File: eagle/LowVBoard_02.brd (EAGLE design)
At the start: 113 x 52.1 mm, 29 parts, among them IC1 ATMEGA328P-PU, IC2 MCP7940M, IC3 SN74HC595, IC4 SN74HC595, J1 CONNJACKR/APCB5.5X2.1MM, Q1 16MHz, Q2 32.768kHz

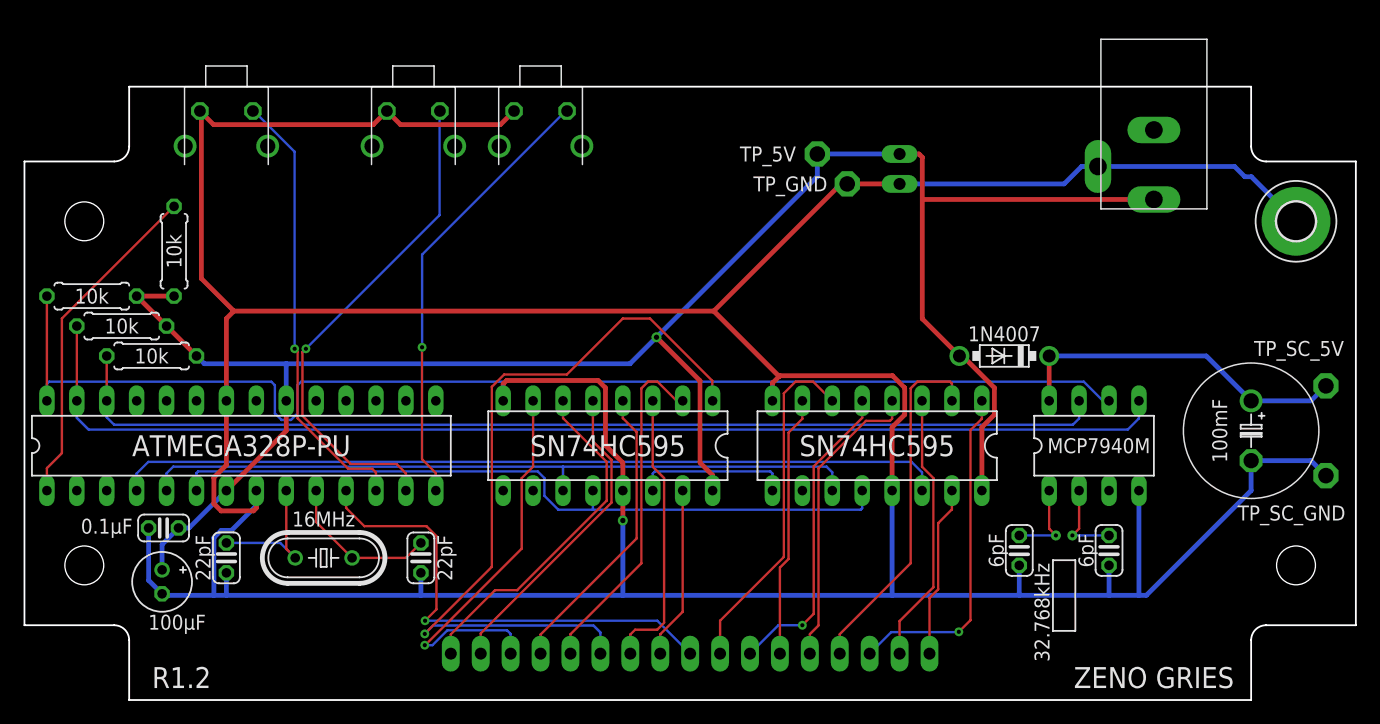
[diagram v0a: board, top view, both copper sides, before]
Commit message: corrected pcb
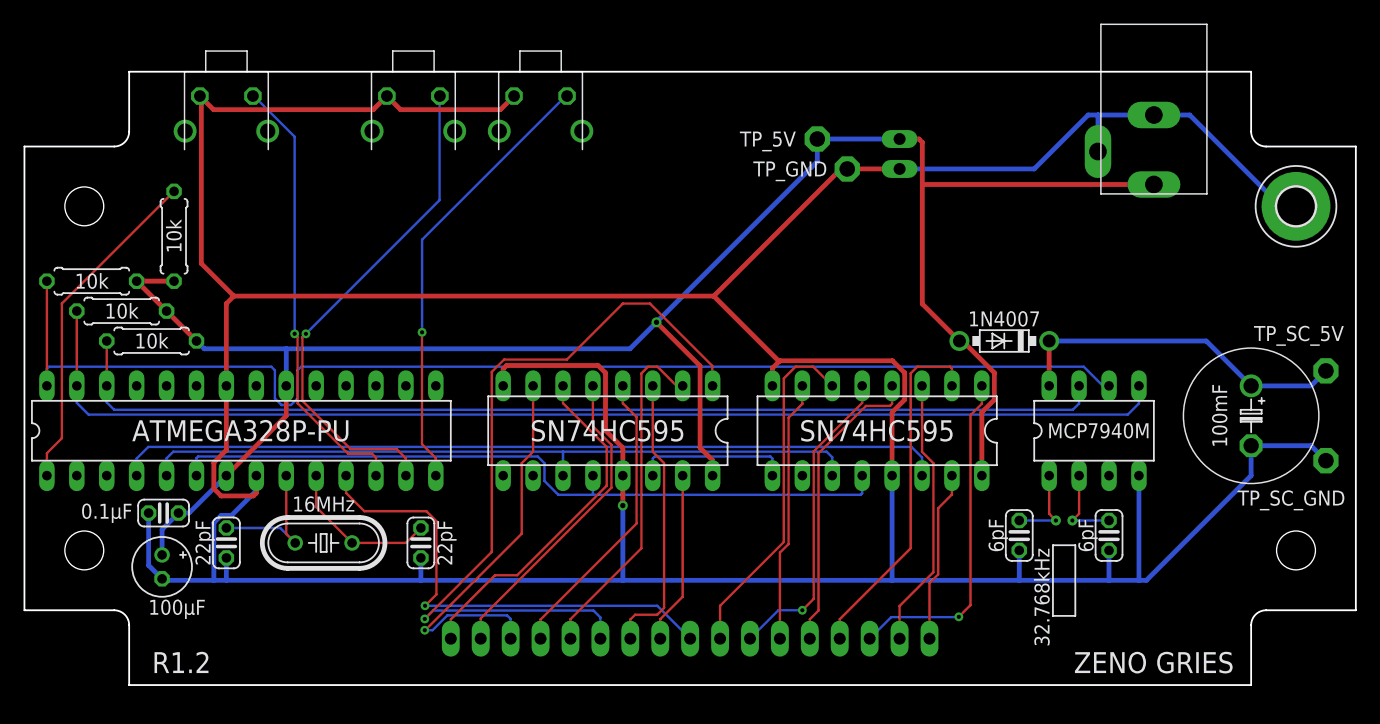
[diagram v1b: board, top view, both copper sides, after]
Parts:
- moved H1 1.27 mm to (108.0, 40.6)
- moved J1 1.27 mm to (95.9, 48.9)
- moved POWER 1.27 mm to (74.3, 45.1)
- moved R1 1.27 mm to (12.7, 38.1)
- moved S1 1.27 mm to (17.1, 48.5)
- moved S2 1.27 mm to (33.0, 48.5)
- moved S3 1.27 mm to (43.8, 48.5)
- moved TP_SC_5V 1.27 mm to (110.5, 26.7)
- moved Q2 1.27 mm to (88.3, 14.0)
- moved DATA 1.27 mm to (56.5, 3.94)
- moved C1 1.27 mm to (11.7, 10.0)
- moved C2 1.27 mm to (11.8, 14.6)
- moved C3 1.27 mm to (33.7, 12.1)
- moved C4 1.27 mm to (17.1, 12.1)
- moved C5 1.27 mm to (92.1, 12.7)
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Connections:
- net GND: now also J1.B
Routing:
- net GND: track 374.8 -> 380.5 mm
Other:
- outline, holes or cut-outs redrawn
